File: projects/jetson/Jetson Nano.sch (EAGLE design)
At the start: 19 parts, among them X1 MKDSN1,5/4-5,08, X2 MKDSN1,5/4-5,08

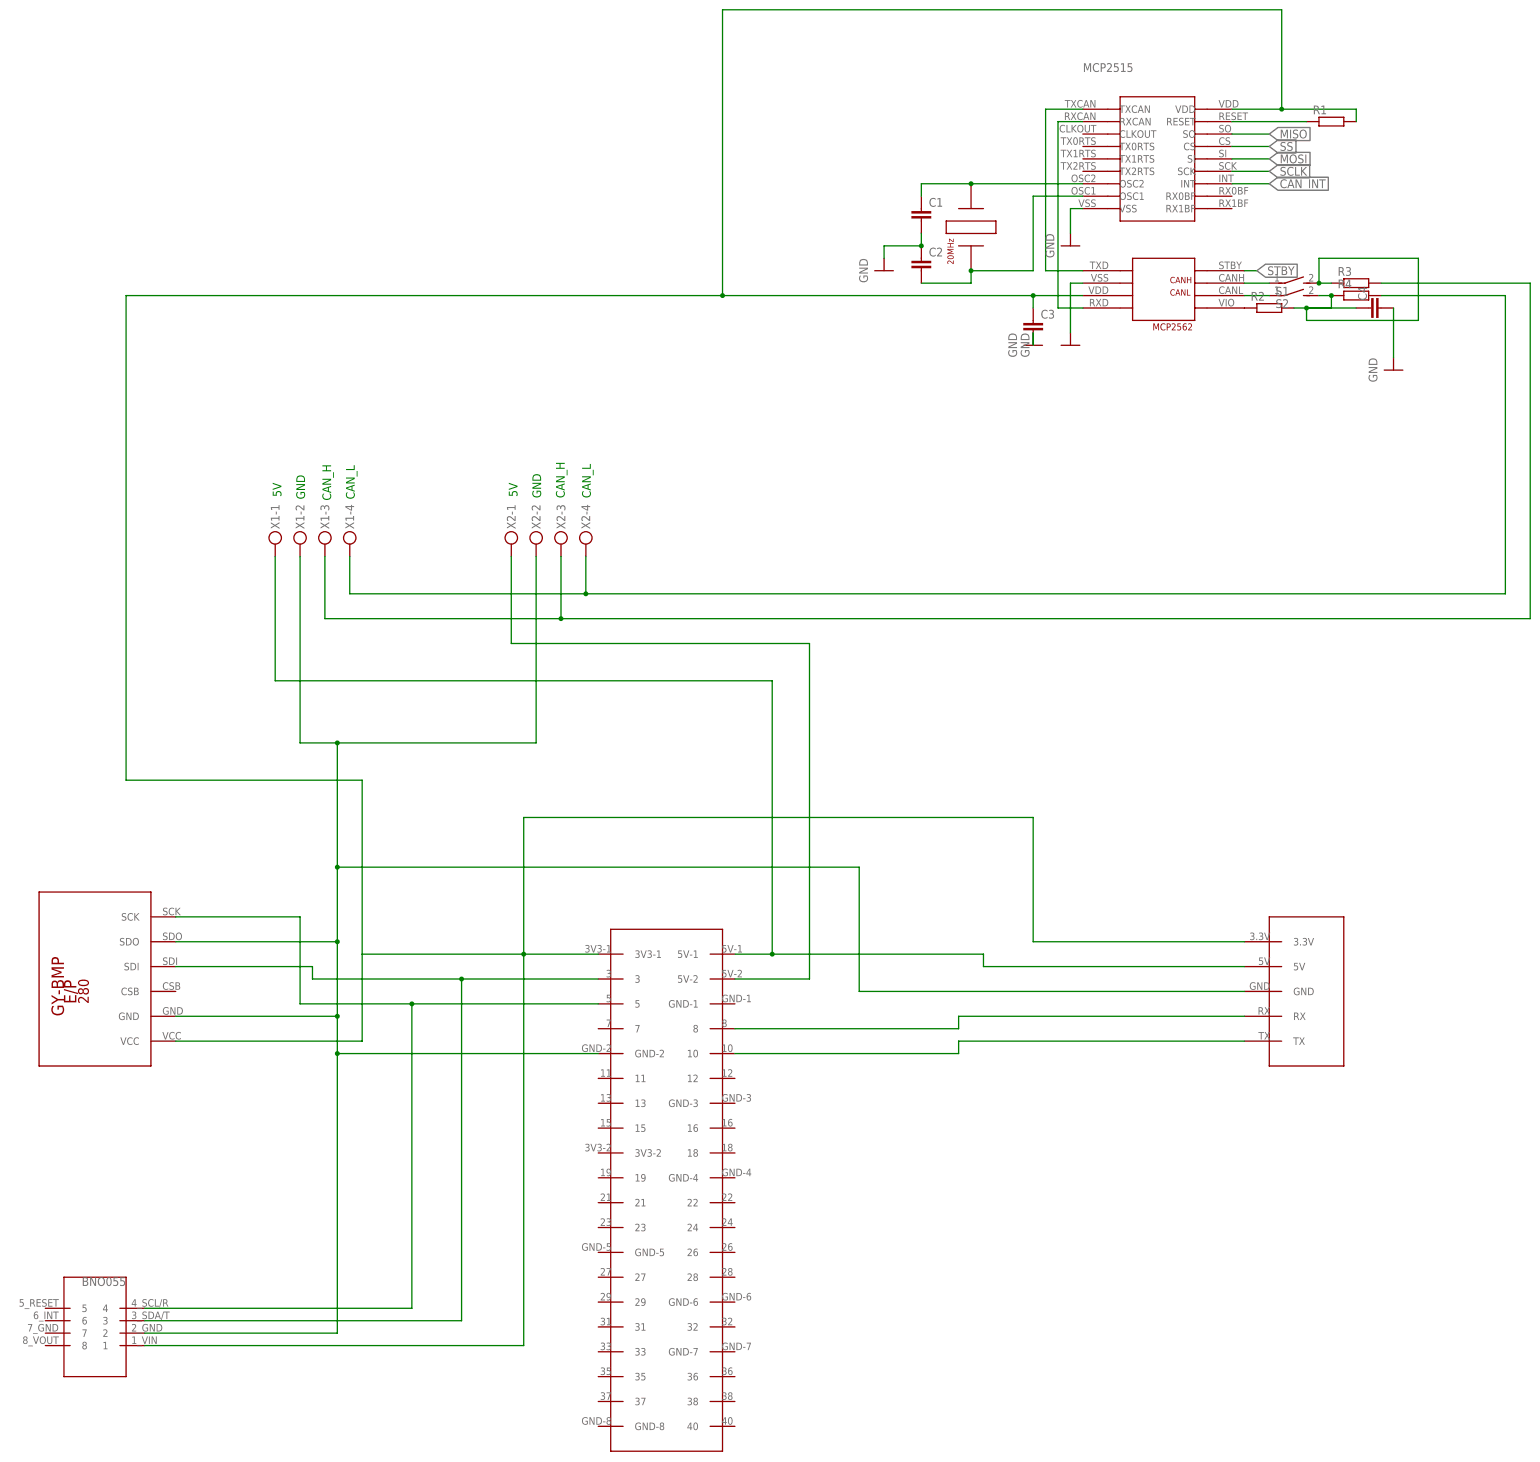
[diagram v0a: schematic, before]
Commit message: change all
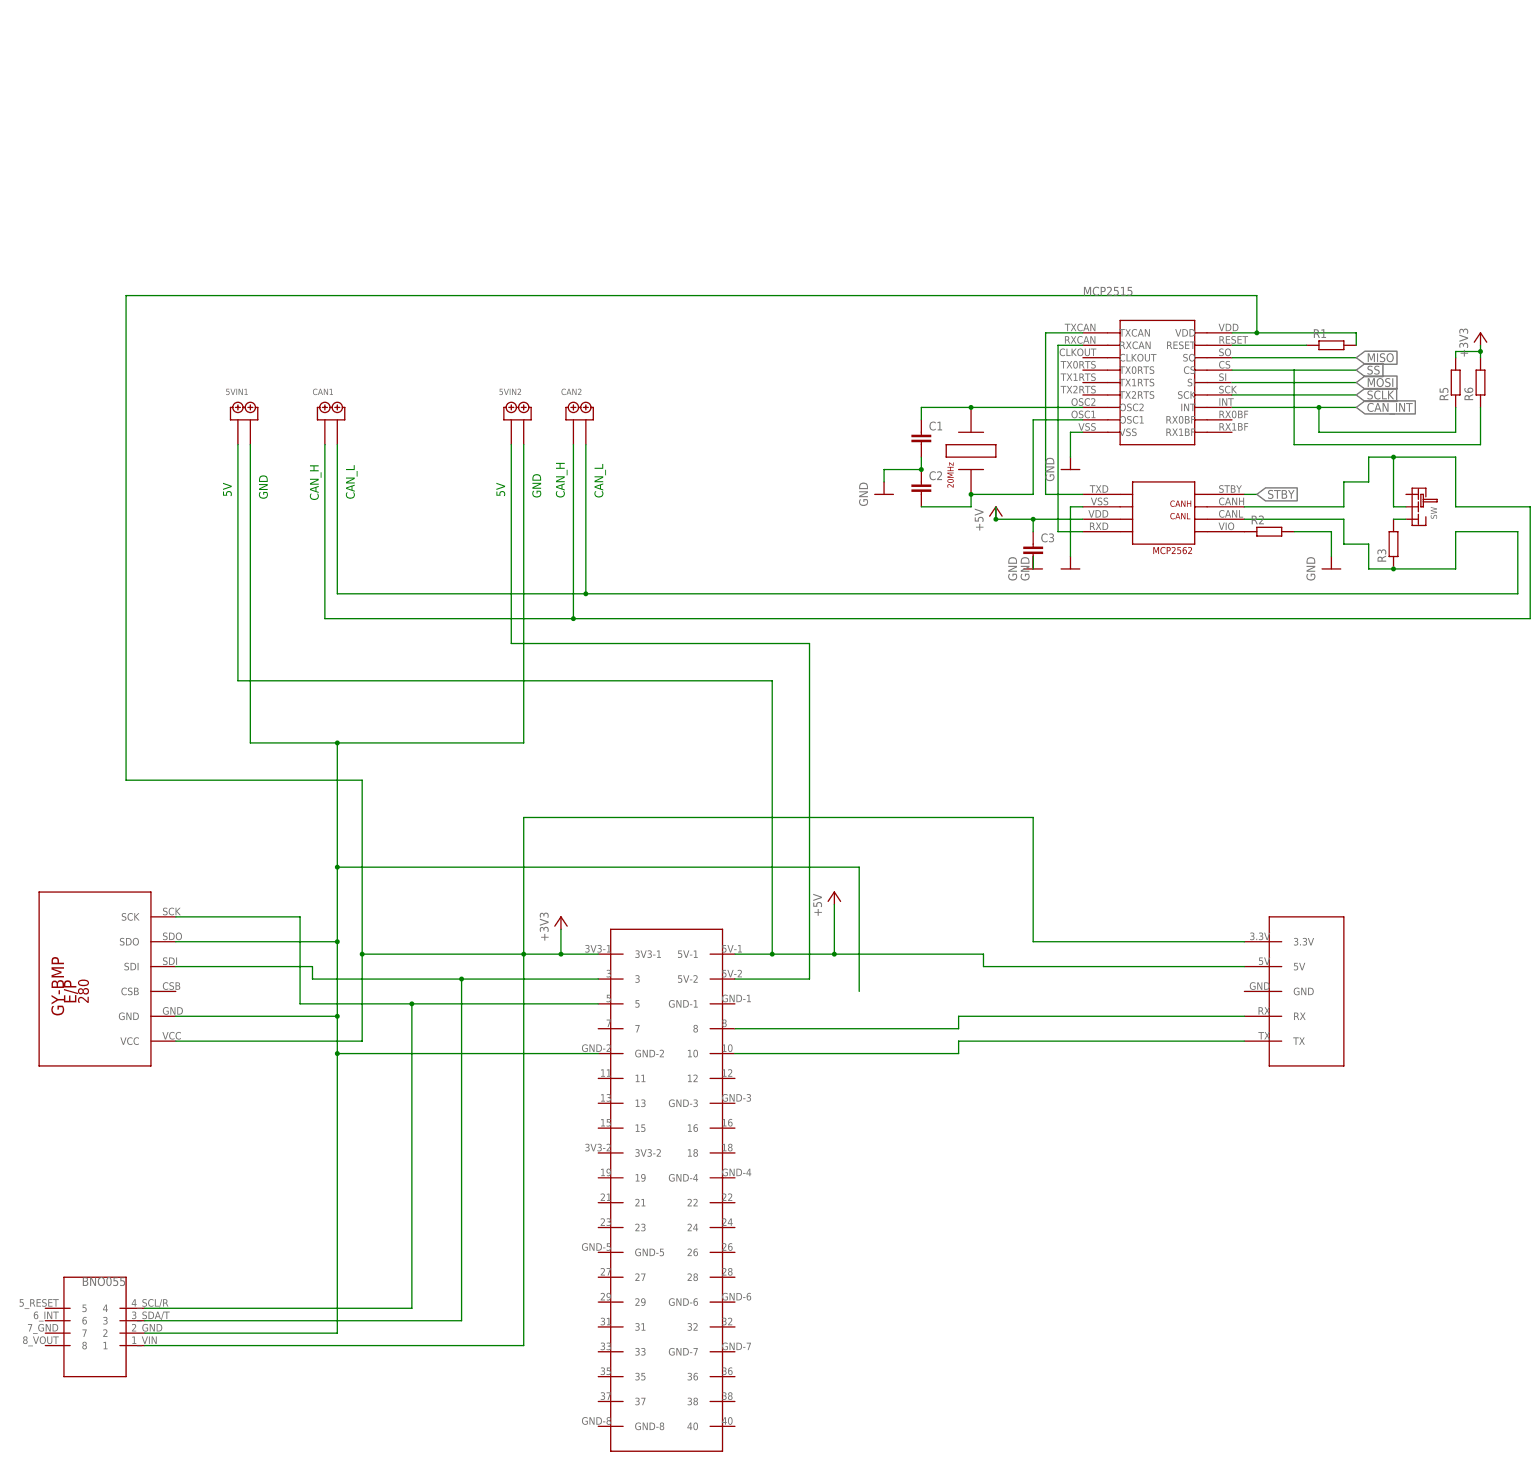
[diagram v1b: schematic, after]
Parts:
- removed C4: (no value), rcl:C-EU025-024X044
- removed R4: (no value), rcl:R-EU_0207/10
- removed S1, S2: (no value), switch-dil:DS01E
- removed X1, X2: MKDSN1,5/4-5,08, con-phoenix-508:MKDSN1,5/4-5,08
- added 5VIN1, 5VIN2, CAN1, CAN2: (no value), TB113-2B-x-x-0-x-x:2PIN
- added R5, R6: (no value), rcl:R-EU_0207/10
- added SW: SRIDE_SWITCH, Sride Switch:SRIDE_SWITCH
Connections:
- removed net 3.3V: C3.1, JN1.3V3-1, MCP1.VDD, R1.2, U$1.VCC, U$2.1, U$3.3.3V, U$4.VDD
- removed net 5V_1: JN1.5V-1, U$3.5V, X1-1.KL
- removed net CAN_H: R3.2, X1-3.KL, X2-3.KL
- removed net CAN_H3: C4.1, R2.2, R3.1, R4.1, S1.2, S2.2
- removed net CAN_L: R4.2, X1-4.KL, X2-4.KL
- new net +3V3: JN1.3V3-1, MCP1.VDD, R1.2, R5.2, R6.2, U$1.VCC, U$2.1, U$3.3.3V
- new net +5V: 5VIN1.P$1, C3.1, JN1.5V-1, U$3.5V, U$4.VDD
- new net N$1: R2.2
- new net N$15: R3.2, SW.R
- net 5V_2: now also 5VIN2.P$1; no longer X2-1.KL
- net CAN_H2: now also CAN1.P$1, CAN2.P$1, SW.LR; no longer S1.1
- net CAN_INT: now also R5.1
- net N$16: now also CAN1.P$2, CAN2.P$2, R3.1; no longer S2.1
- net N$2: now also 5VIN1.P$2, 5VIN2.P$2; no longer U$3.GND, X1-2.KL, X2-2.KL
- net SS: now also R6.1
- net V-: no longer C4.2
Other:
- moved on the sheet: C1, C2, C3, R1, R2, R3
